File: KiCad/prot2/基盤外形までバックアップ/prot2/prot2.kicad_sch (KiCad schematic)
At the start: 193 parts, among them J1 Conn_01x02_Socket, J2 LED_SW, J3 Conn_01x04_Socket, Q1 Q_Photo_NPN, Q10 Q_Photo_NPN, Q11 Q_Photo_NPN, Q12 Q_Photo_NPN, Q13 Q_Photo_NPN, Q14 Q_Photo_NPN, Q15 Q_Photo_NPN, Q16 Q_Photo_NPN, Q17 Q_Photo_NPN, Q18 Q_Photo_NPN, Q19 Q_Photo_NPN, Q2 Q_Photo_NPN, Q20 Q_Photo_NPN, Q21 Q_Photo_NPN, Q22 Q_Photo_NPN, Q23 Q_Photo_NPN, Q24 Q_Photo_NPN, Q25 Q_Photo_NPN, Q26 Q_Photo_NPN, Q27 Q_Photo_NPN, Q28 Q_Photo_NPN, Q29 Q_Photo_NPN, Q3 Q_Photo_NPN, Q30 Q_Photo_NPN, Q31 Q_Photo_NPN, Q32 Q_Photo_NPN, Q4 Q_Photo_NPN, Q5 Q_Photo_NPN, Q6 Q_Photo_NPN, Q7 Q_Photo_NPN, Q8 Q_Photo_NPN, Q9 Q_Photo_NPN, U1 LM339, U2 LM339, U3 LM339, U4 LM339, U5 LM339, U6 LM339, U7 LM339, U8 LM339

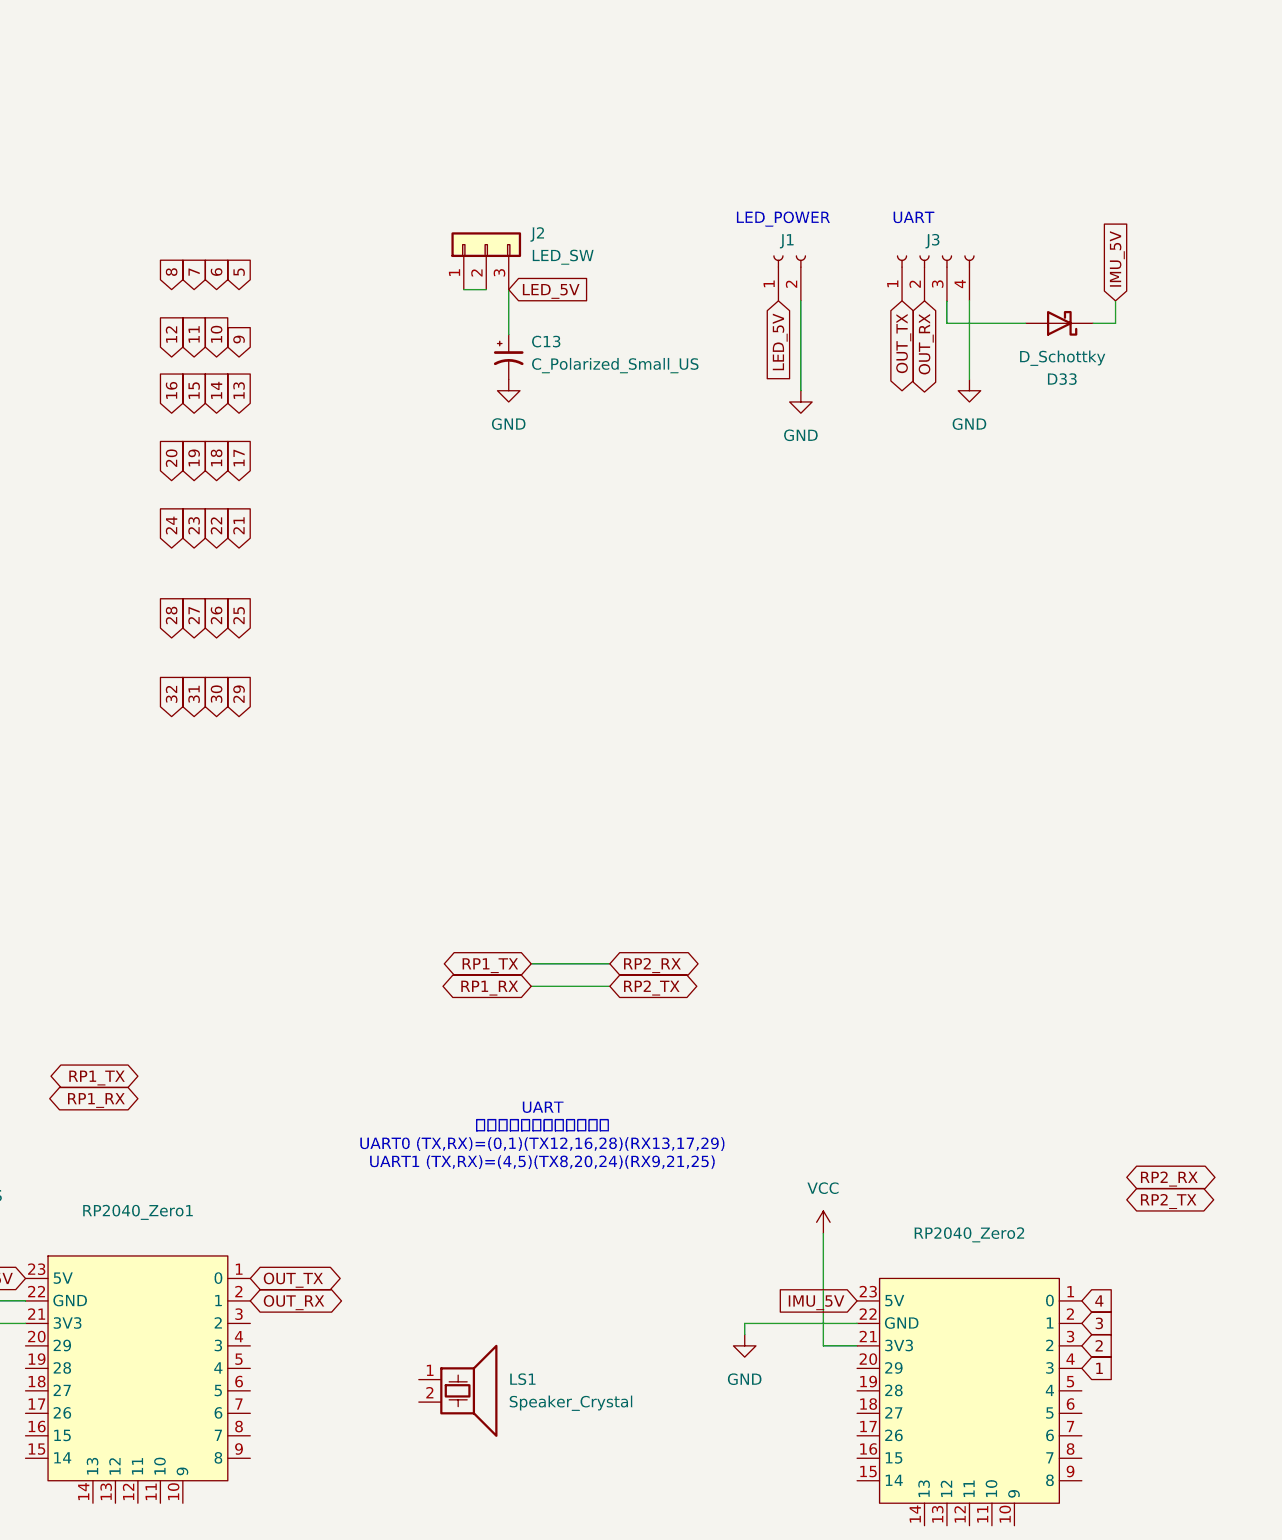
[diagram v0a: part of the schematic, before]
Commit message: 外形まで完成くそ
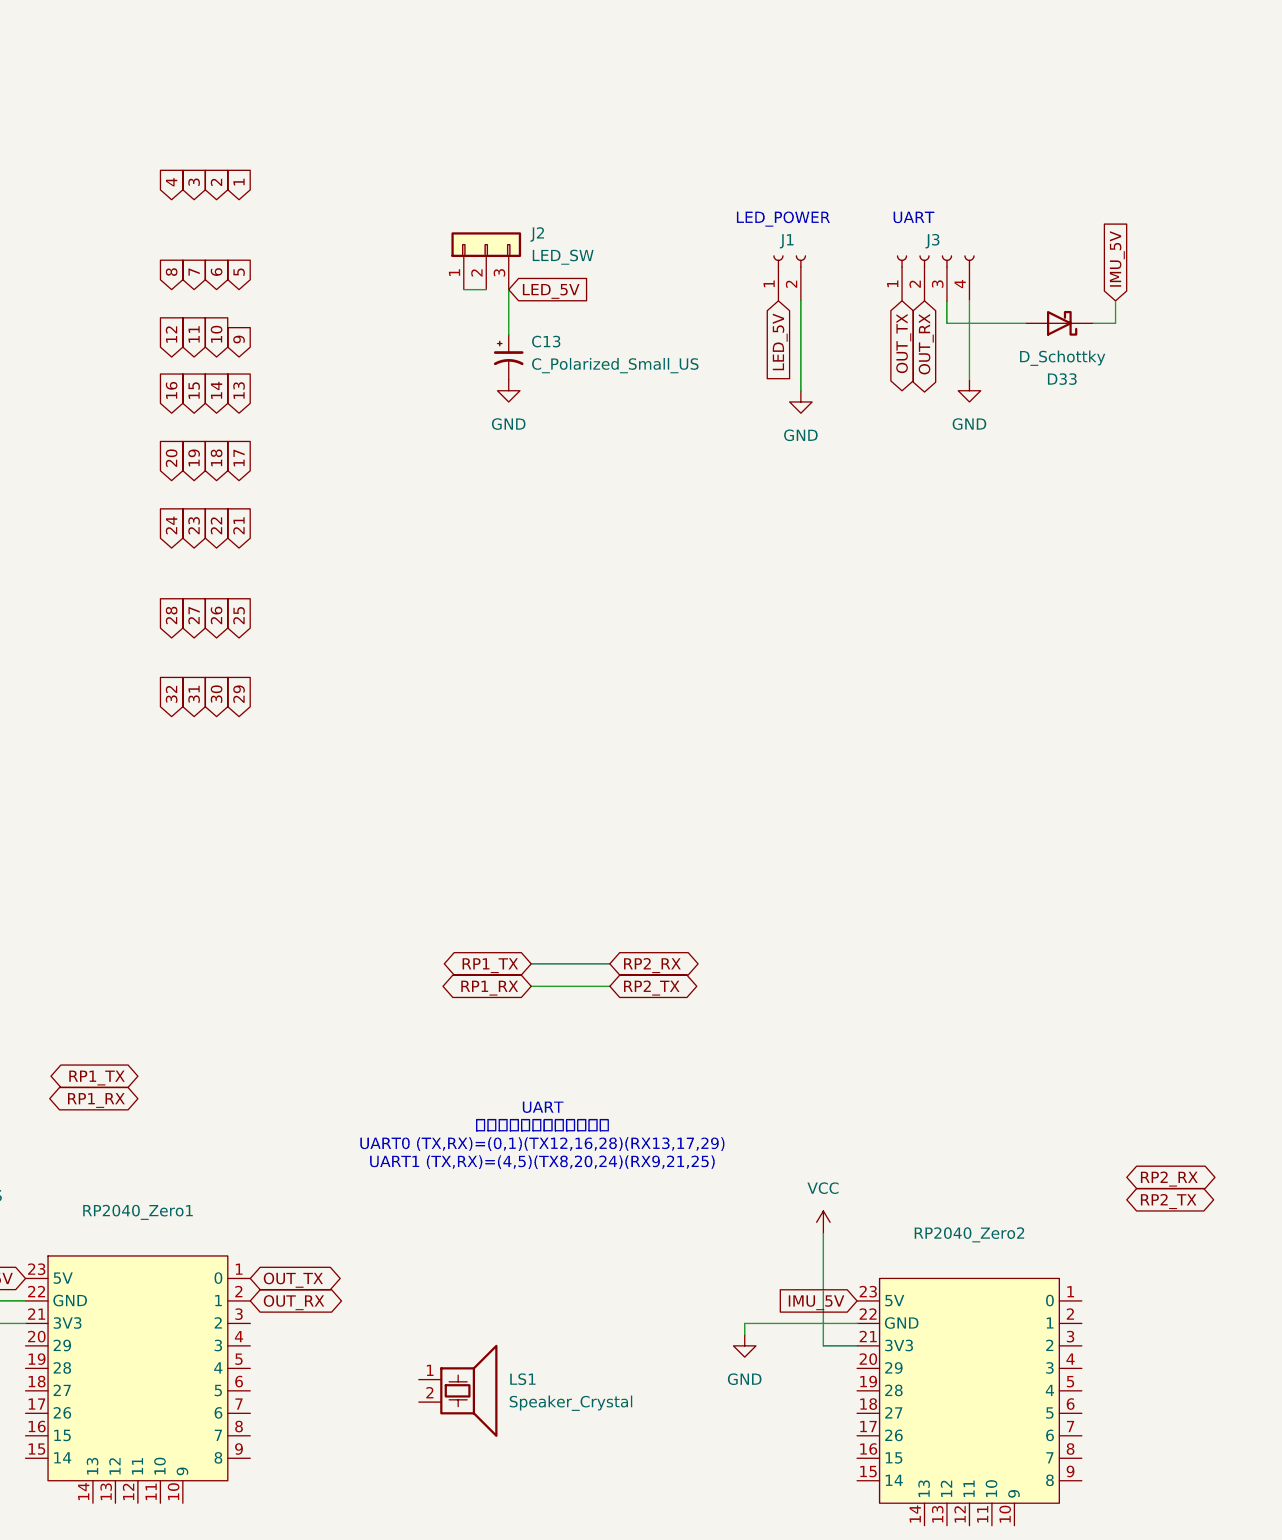
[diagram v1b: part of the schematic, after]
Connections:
- net 1: no longer RP2040_Zero2.4 (3)
- net 2: no longer RP2040_Zero2.3 (2)
- net 3: no longer RP2040_Zero2.2 (1)
- net 4: no longer RP2040_Zero2.1 (0)
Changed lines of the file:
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@@
 	(global_label "2"
 		(shape input)
-		(at 207.01 294.64 0)
-		(fields_autoplaced yes)
-		(effects
-			(font
-				(size 1.27 1.27)
-			)
-			(justify left)
-		)
-		(property "Intersheetrefs" "${INTERSHEET_REFS}"
-			(at 211.2047 294.64 0)
+		(at 109.22 165.1 90)
+		(fields_autoplaced yes)
+		(effects
+			(font
+				(size 1.27 1.27)
+			)
+			(justify left)
+		)
+		(property "Intersheetrefs" "${INTERSHEET_REFS}"
+			(at 109.22 160.9053 90)
 			(effects
 				(font
@@
 	(global_label "4"
 		(shape input)
-		(at 207.01 289.56 0)
-		(fields_autoplaced yes)
-		(effects
-			(font
-				(size 1.27 1.27)
-			)
-			(justify left)
-		)
-		(property "Intersheetrefs" "${INTERSHEET_REFS}"
-			(at 211.2047 289.56 0)
+		(at 104.14 165.1 90)
+		(fields_autoplaced yes)
+		(effects
+			(font
+				(size 1.27 1.27)
+			)
+			(justify left)
+		)
+		(property "Intersheetrefs" "${INTERSHEET_REFS}"
+			(at 104.14 160.9053 90)
 			(effects
 				(font
@@
 	(global_label "3"
 		(shape input)
-		(at 207.01 292.1 0)
-		(fields_autoplaced yes)
-		(effects
-			(font
-				(size 1.27 1.27)
-			)
-			(justify left)
-		)
-		(property "Intersheetrefs" "${INTERSHEET_REFS}"
-			(at 211.2047 292.1 0)
+		(at 106.68 165.1 90)
+		(fields_autoplaced yes)
+		(effects
+			(font
+				(size 1.27 1.27)
+			)
+			(justify left)
+		)
+		(property "Intersheetrefs" "${INTERSHEET_REFS}"
+			(at 106.68 160.9053 90)
 			(effects
 				(font
@@
 	(global_label "1"
 		(shape input)
-		(at 207.01 297.18 0)
-		(fields_autoplaced yes)
-		(effects
-			(font
-				(size 1.27 1.27)
-			)
-			(justify left)
-		)
-		(property "Intersheetrefs" "${INTERSHEET_REFS}"
-			(at 211.2047 297.18 0)
-			(effects
-				(font
+		(at 111.76 165.1 90)
+		(fields_autoplaced yes)
+		(effects
+			(font
+				(size 1.27 1.27)
+			)
+			(justify left)
+		)
+		(property "Intersheetrefs" "${INTERSHEET_REFS}"
+			(at 111.76 160.9053 90)
+			(effects
+				(font
